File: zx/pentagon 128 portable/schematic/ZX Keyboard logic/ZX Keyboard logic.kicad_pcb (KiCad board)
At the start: 2 copper layers, 99 x 66 mm, 51 parts, among them IC1 SN74LS245DW, IC2 SN74LS27N, IC3 SN74LS245DW, J1 Conn_01x03, J2 Conn_01x14, J3 Conn_01x02

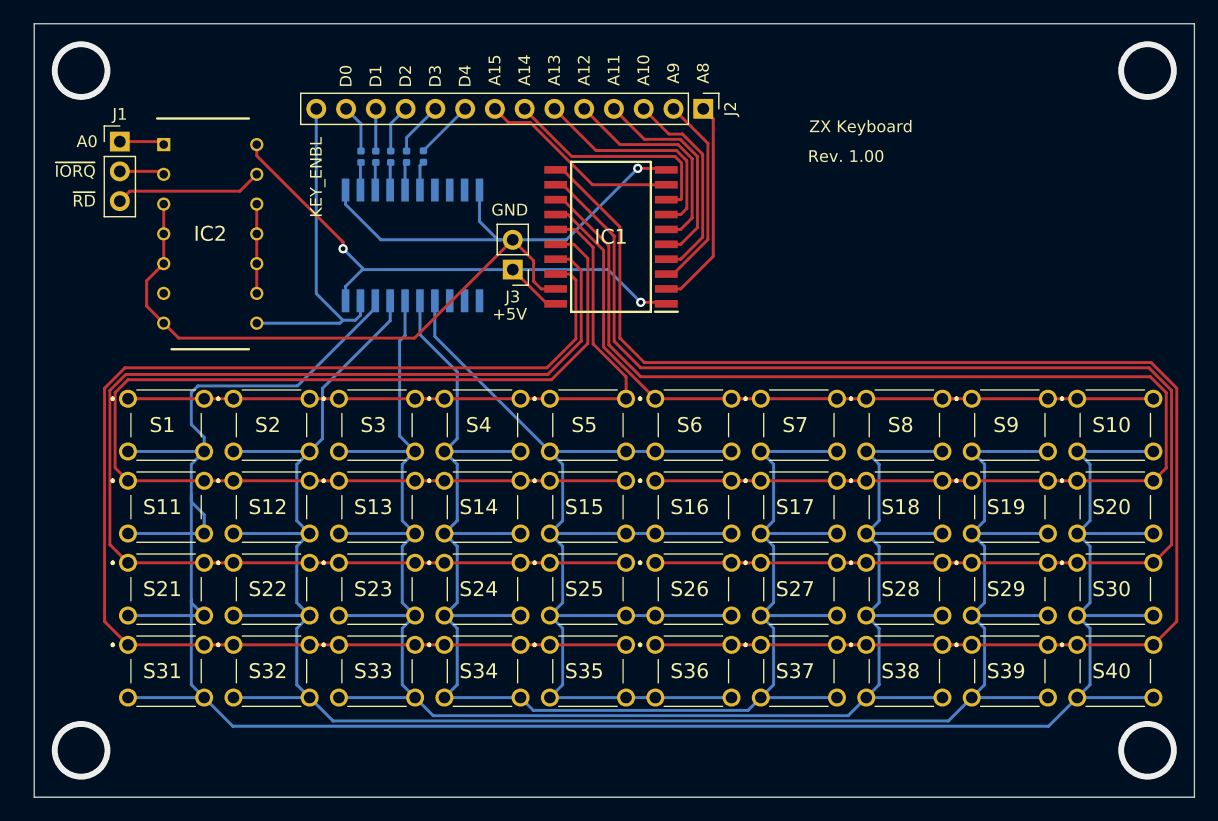
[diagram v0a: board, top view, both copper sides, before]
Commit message: fixed keyboard
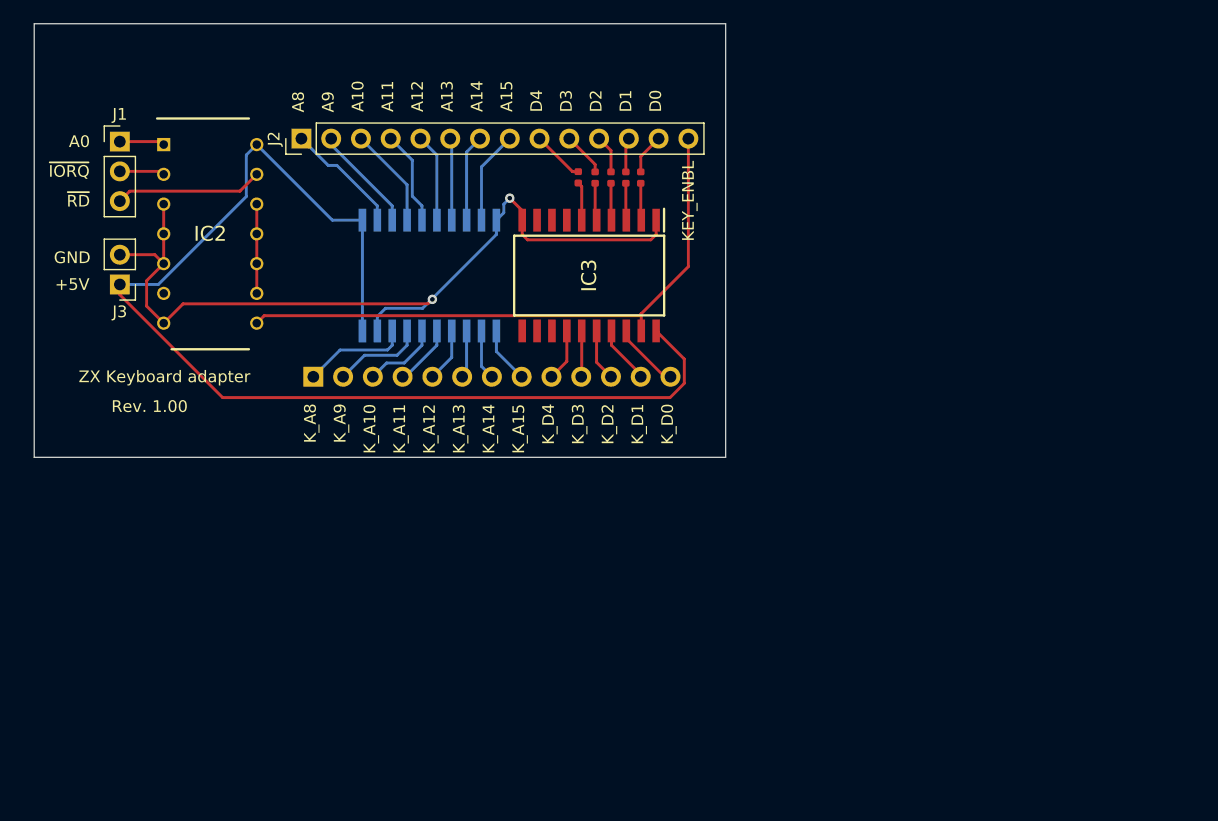
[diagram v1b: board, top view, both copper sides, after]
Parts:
- removed S1: 1, SamacSys_Parts:118259104
- removed S10: 0, SamacSys_Parts:118259104
- removed S11: Q, SamacSys_Parts:118259104
- removed S12: W, SamacSys_Parts:118259104
- removed S13: E, SamacSys_Parts:118259104
- removed S14: R, SamacSys_Parts:118259104
- removed S15: T, SamacSys_Parts:118259104
- removed S16: Y, SamacSys_Parts:118259104
- removed S17: U, SamacSys_Parts:118259104
- removed S18: I, SamacSys_Parts:118259104
- removed S19: O, SamacSys_Parts:118259104
- removed S2: 2, SamacSys_Parts:118259104
- removed S20: P, SamacSys_Parts:118259104
- removed S21: A, SamacSys_Parts:118259104
- removed S22: S, SamacSys_Parts:118259104
- removed S23: D, SamacSys_Parts:118259104
- removed S24: F, SamacSys_Parts:118259104
- removed S25: G, SamacSys_Parts:118259104
- removed S26: H, SamacSys_Parts:118259104
- removed S27: J, SamacSys_Parts:118259104
- removed S28: K, SamacSys_Parts:118259104
- removed S29: L, SamacSys_Parts:118259104
- removed S3: 3, SamacSys_Parts:118259104
- removed S30: ENTER, SamacSys_Parts:118259104
- removed S31: CAPS, SamacSys_Parts:118259104
- removed S32: Z, SamacSys_Parts:118259104
- removed S33: X, SamacSys_Parts:118259104
- removed S34: C, SamacSys_Parts:118259104
- removed S35: V, SamacSys_Parts:118259104
- removed S36: B, SamacSys_Parts:118259104
- removed S37: N, SamacSys_Parts:118259104
- removed S38: M, SamacSys_Parts:118259104
- removed S39: SYMB, SamacSys_Parts:118259104
- removed S4: 4, SamacSys_Parts:118259104
- removed S40: SPACE, SamacSys_Parts:118259104
- removed S5: 5, SamacSys_Parts:118259104
- removed S6: 6, SamacSys_Parts:118259104
- removed S7: 7, SamacSys_Parts:118259104
- removed S8: 8, SamacSys_Parts:118259104
- removed S9: 9, SamacSys_Parts:118259104
- added J4: Conn_01x13, Connector_PinSocket_2.54mm:PinSocket_1x13_P2.54mm_Vertical, B.Cu at (51.8, 103.1)
- IC1: moved to B.Cu
- IC3, R1, R2, R3, R4, R?-R1: moved to F.Cu
- moved J2 34.4 mm to (50.8, 82.8), turned to 90 degrees
- moved J3 33.6 mm to (35.3, 95.2)
- moved R?-R1 23.9 mm to (79.8, 86.1)
- moved R1 21.4 mm to (78.5, 86.1)
- moved R2 18.9 mm to (77.2, 86.1)
- moved R3 16.2 mm to (75.9, 86.1)
- moved IC1 15.8 mm to (61.7, 94.5), turned to 270 degrees
- moved IC3 15.3 mm to (75.4, 94.5)
- moved R4 13.3 mm to (74.4, 86.1)
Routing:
- net /K_D0: track 204.4 -> 6.38 mm
- net /K_D1: track 173.3 -> 4.95 mm
- net /K_D2: track 152.8 -> 4.42 mm
- net /K_D3: track 135.5 -> 3.99 mm
- net /K_A15: track 131.5 -> 4.81 mm
- net /K_A14: track 122.9 -> 4.28 mm
- net /K_A13: track 114.4 -> 4.07 mm
- net /K_A8: track 114.2 -> 9.07 mm
- net /K_A9: track 108.4 -> 7.80 mm
- net /K_D4: track 102.6 -> 4.45 mm
- net /K_A10: track 103.1 -> 6.53 mm
- net /K_A12: track 62.4 -> 4.59 mm
- net /K_A11: track 60.4 -> 5.26 mm
- net +5V: track 49.7 -> 98.5 mm, vias 2 -> 0
- net /KEY_ENBL: track 29.3 -> 51.2 mm
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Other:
- board size 99 x 66 mm -> 59 x 37 mm
- board text added: "K_A10"
- board text added: "K_A11"
- board text added: "K_A12"
- board text added: "K_A13"
- board text added: "K_A14"
- board text added: "K_A15"
- board text added: "K_A8"
- board text added: "K_A9"
- board text added: "K_D0"
- board text added: "K_D1"
- board text added: "K_D2"
- board text added: "K_D3"
- board text added: "K_D4"
- board text added: "ZX Keyboard adapter"
- board text removed: "ZX Keyboard"
